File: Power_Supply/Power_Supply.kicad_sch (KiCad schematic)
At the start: 29 parts, among them J1 Cable_PAD, J2 Cable_PAD, J3 CONN_01X03, J4 CONN_01X03, J5 jack, Q1 TIP41C, Q2 BD139, Q3 BC548, Q4 BC558, Q5 BC558, U1 LM358

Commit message: new footprint
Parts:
- Q1: footprint EESTN5:TO-220 -> Modified_Footprints:TO-220-3_Vertical
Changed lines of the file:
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@@
 			)
 		)
-		(property "Footprint" "EESTN5:TO-220"
+		(property "Footprint" "Modified_Footprints:TO-220-3_Vertical"
 			(at 176.53 168.58 0)
 			(effects

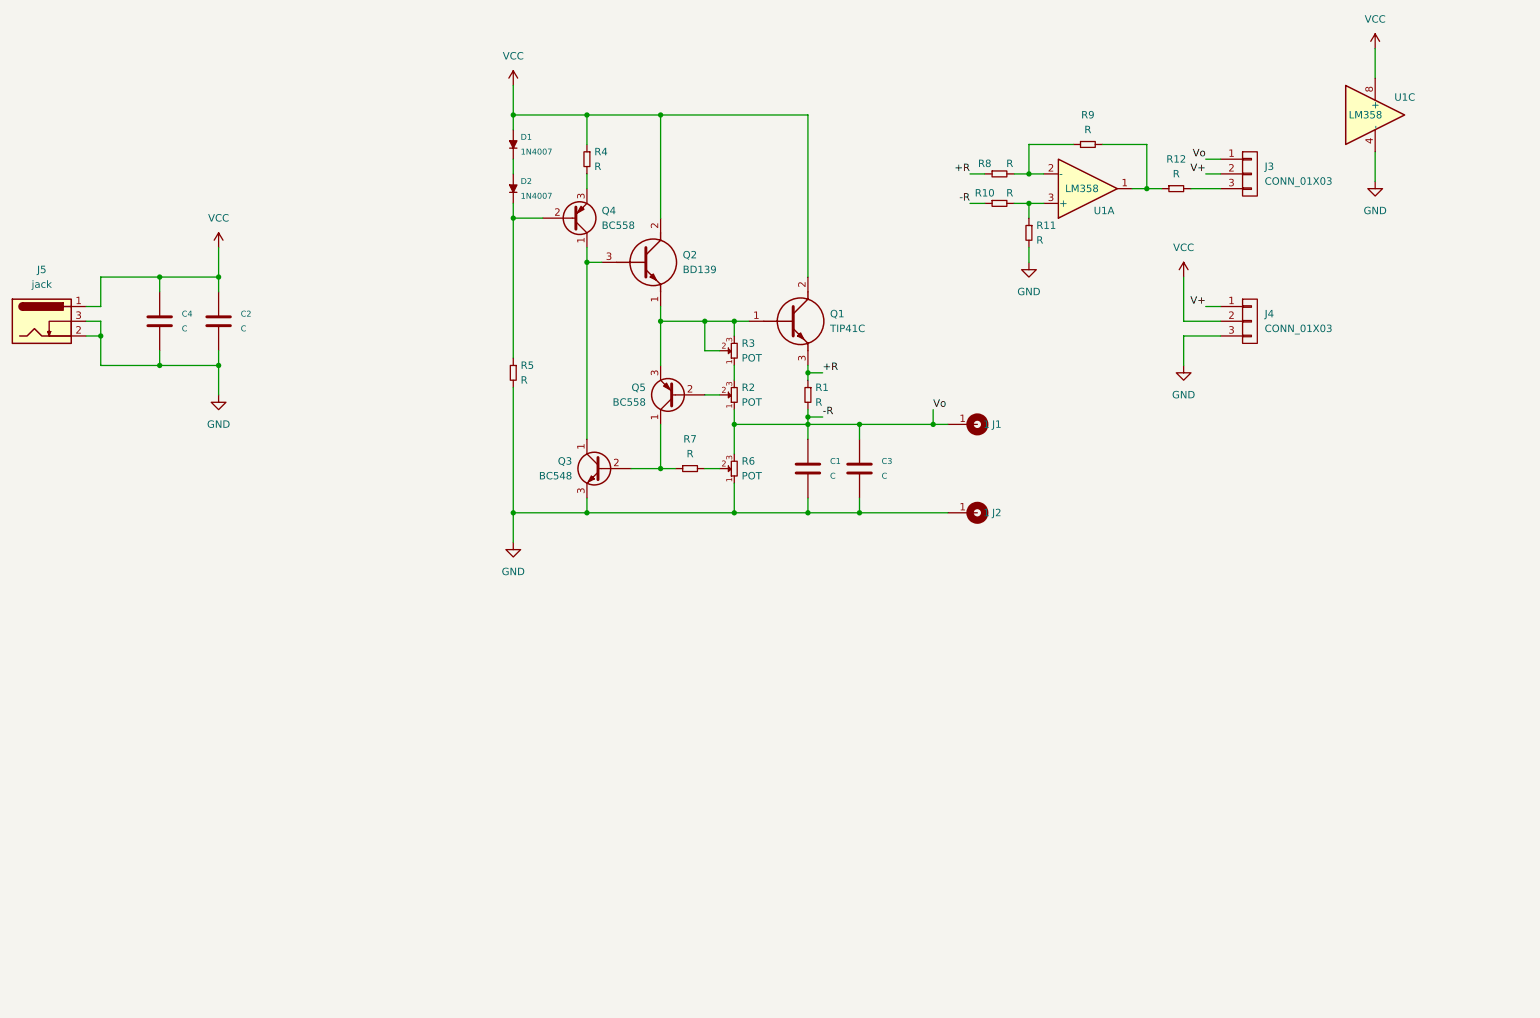
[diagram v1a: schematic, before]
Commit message: new
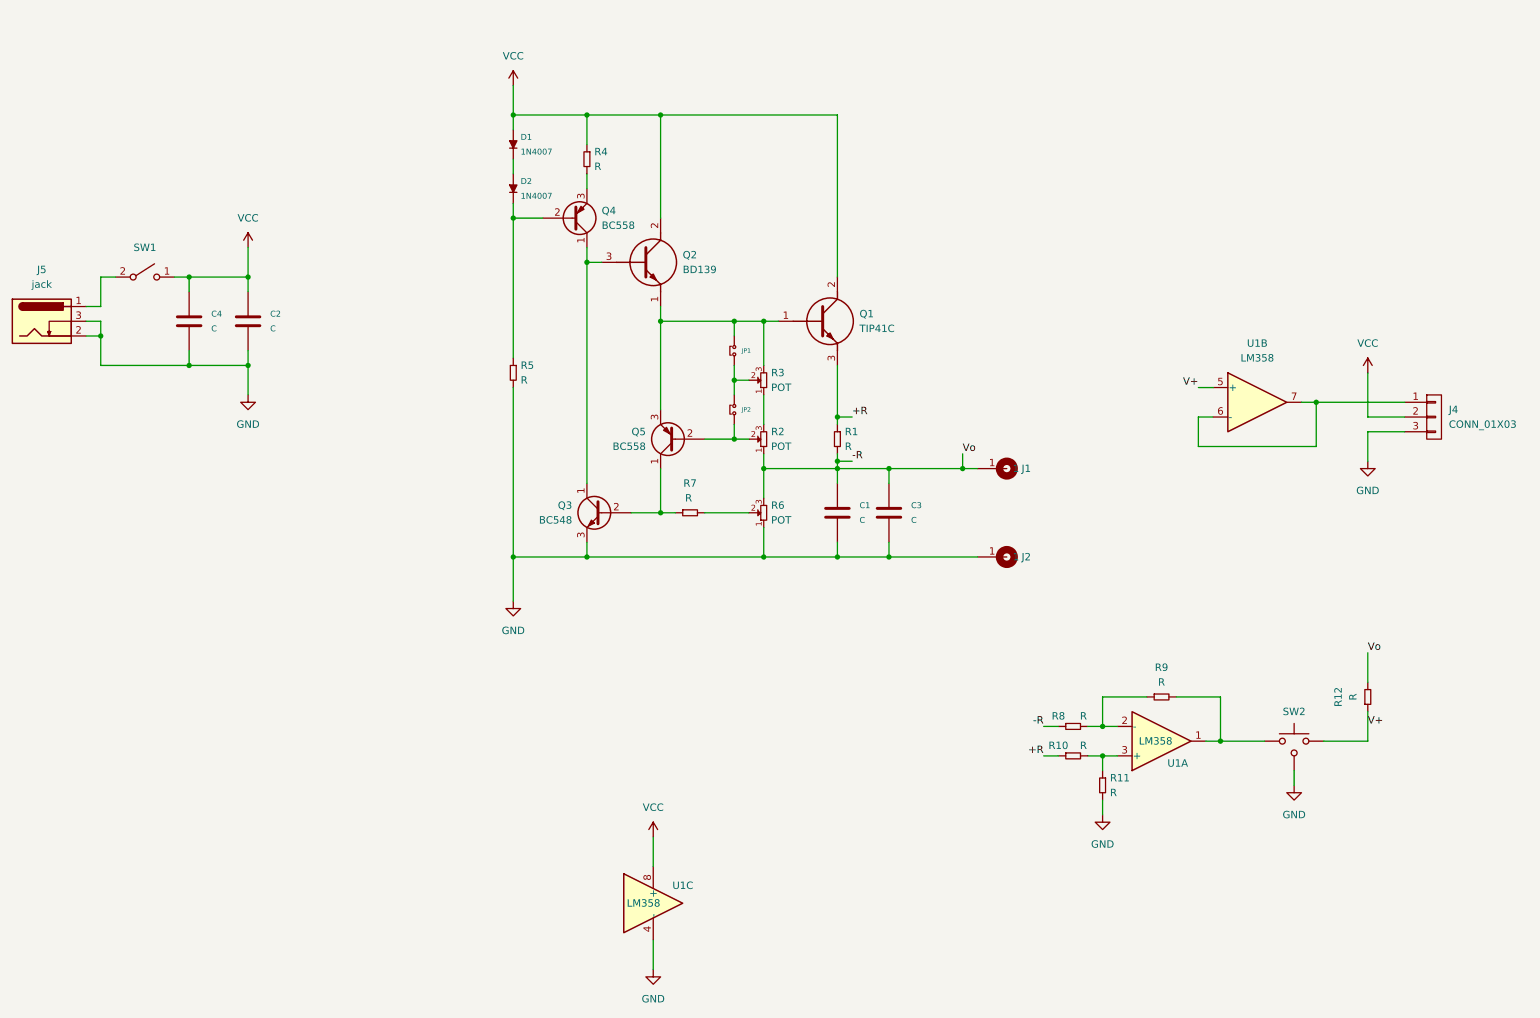
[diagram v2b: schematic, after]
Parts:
- removed J3: CONN_01X03, EESTN5:Pin_Header_3, symbol EESTN5:CONN_01X03
- added JP1, JP2: Jumper, symbol EESTN5:Jumper
- added SW1: SW_SPST, symbol SW:SW_SPST
- added SW2: SW_Push, symbol SW:SW_Push
- added unit 2 of U1
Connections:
- net +R: now also R10.1; no longer R8.1
- net -R: now also R12.2, R8.1; no longer R10.1
- net GND: now also SW2.3
- net V+: now also R12.1, SW2.2, U1.5 (+); no longer J4.1 (P1)
- net VCC: now also SW1.1 (A); no longer J5.1
- net at R9.2, U1.1: now also SW2.1; no longer R12.1
- net at Q1.1 (B), Q2.1 (E), Q5.3 (E)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: now also JP1.1 (A); no longer R3.2
- net at Q5.2 (B), R2.2: now also JP2.2 (B)
- new net: JP1.2 (B), JP2.1 (A), R3.2
- new net: J4.1 (P1), U1.6 (-), U1.7
- new net: J5.1, SW1.2 (B)
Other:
- moved on the sheet: C1, C2, C3, C4, J1, J2, J4, Q1, Q3, Q5, R1, R10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
